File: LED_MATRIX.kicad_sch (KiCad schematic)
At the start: 17 parts, among them J1 Conn_01x01, J2 Conn_01x01, U1 AS1115-BSST, U2 TLC5940PWP

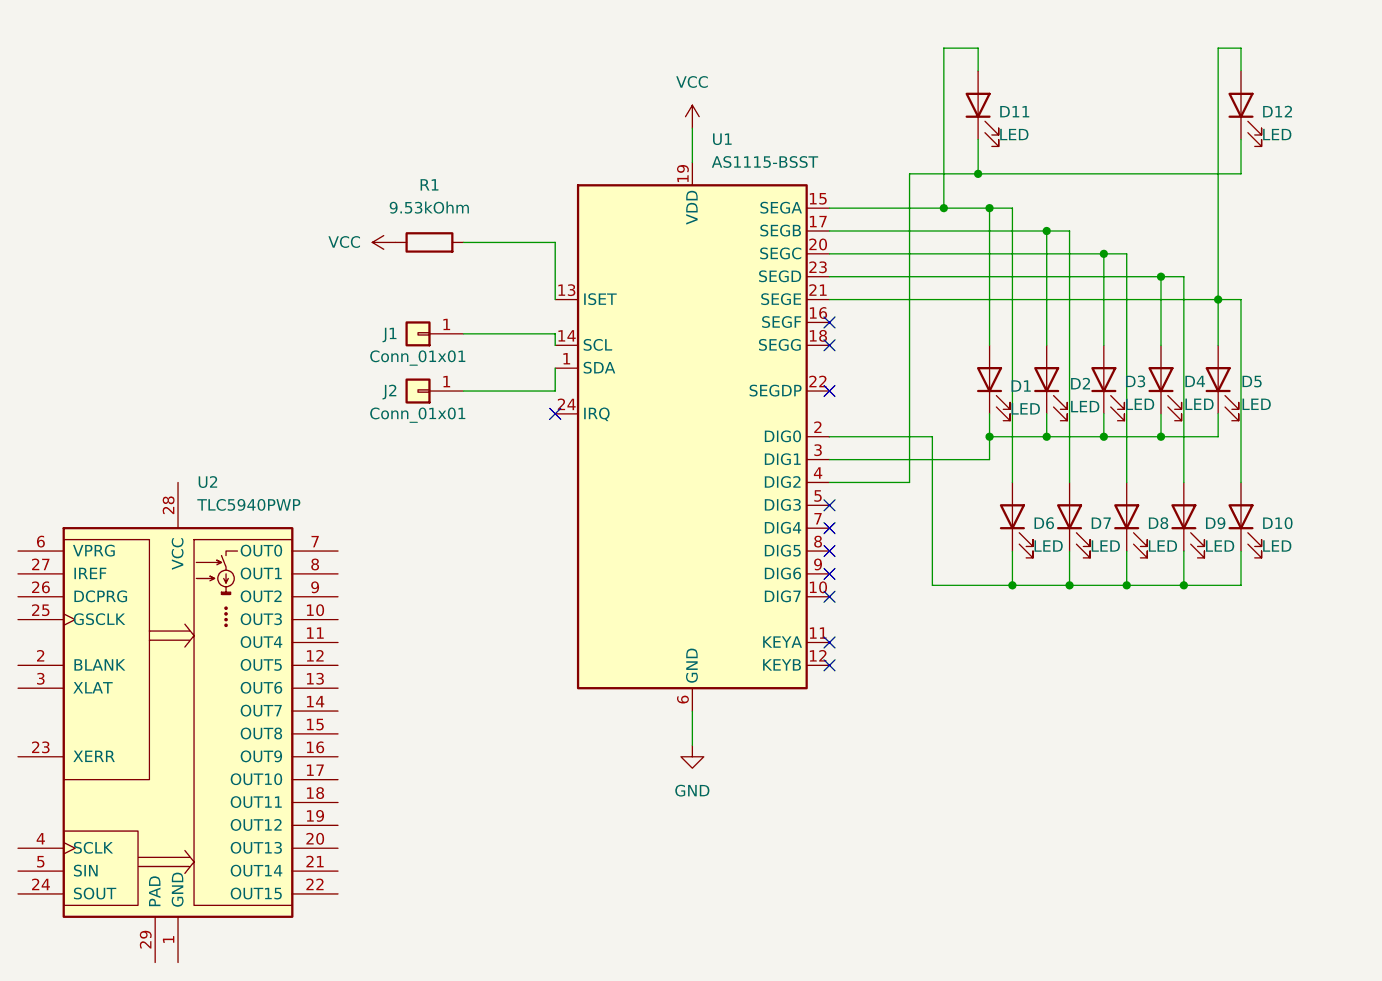
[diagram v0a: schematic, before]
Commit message: wip
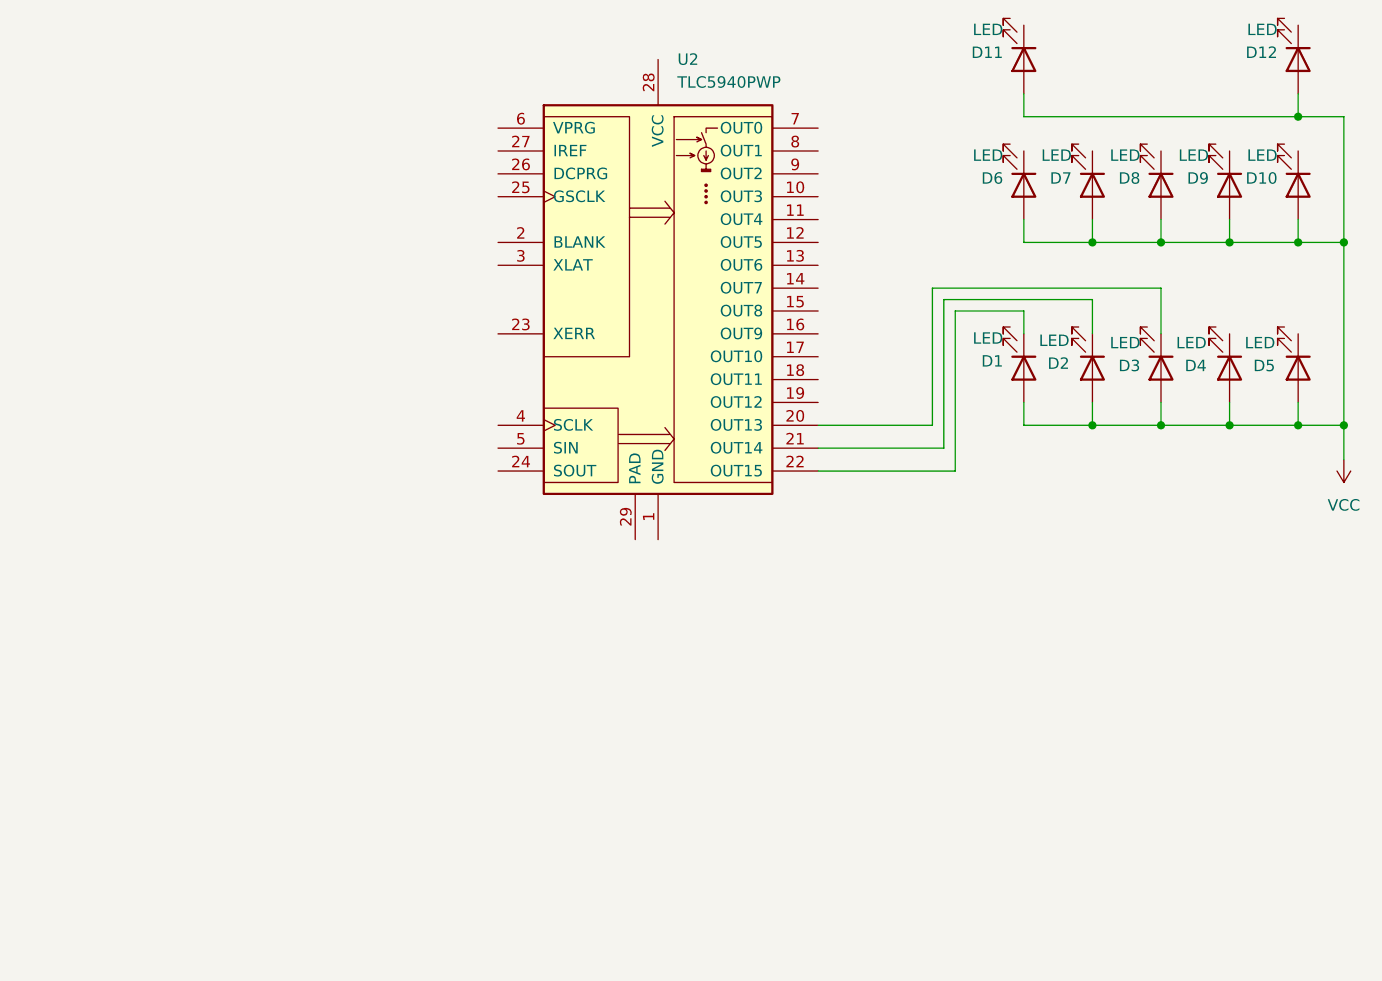
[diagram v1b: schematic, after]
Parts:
- removed J1, J2: Conn_01x01, TestPoint:TestPoint_THTPad_2.0x2.0mm_Drill1.0mm, symbol Connector_Generic:Conn_01x01
- removed R1: 9.53kOhm, Resistor_SMD:R_0805_2012Metric_Pad1.20x1.40mm_HandSolder, symbol Device:R
- removed U1: AS1115-BSST, Package_SO:QSOP-24_3.9x8.7mm_P0.635mm, symbol Interface_Expansion:AS1115-BSST
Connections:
- net VCC: now also D1.2 (A), D10.2 (A), D11.2 (A), D12.2 (A), D2.2 (A), D3.2 (A), D4.2 (A), D5.2 (A), D6.2 (A), D7.2 (A), D8.2 (A), D9.2 (A)
- net at D12.1 (K): no longer D11.1 (K)
- net at U2.20 (OUT13): now also D3.1 (K)
- net at U2.21 (OUT14): now also D2.1 (K)
- net at U2.22 (OUT15): now also D1.1 (K)
- now unconnected: D10.1 (K), D4.1 (K), D5.1 (K), D6.1 (K), D7.1 (K), D8.1 (K), D9.1 (K)
- no-connect marks 11 -> 0
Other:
- moved on the sheet: D1, D10, D11, D12, D2, D3, D4, D5, D6, D7, D8, D9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
